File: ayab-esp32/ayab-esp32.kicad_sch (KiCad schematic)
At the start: 22 parts, among them U101 SN74LVC4245

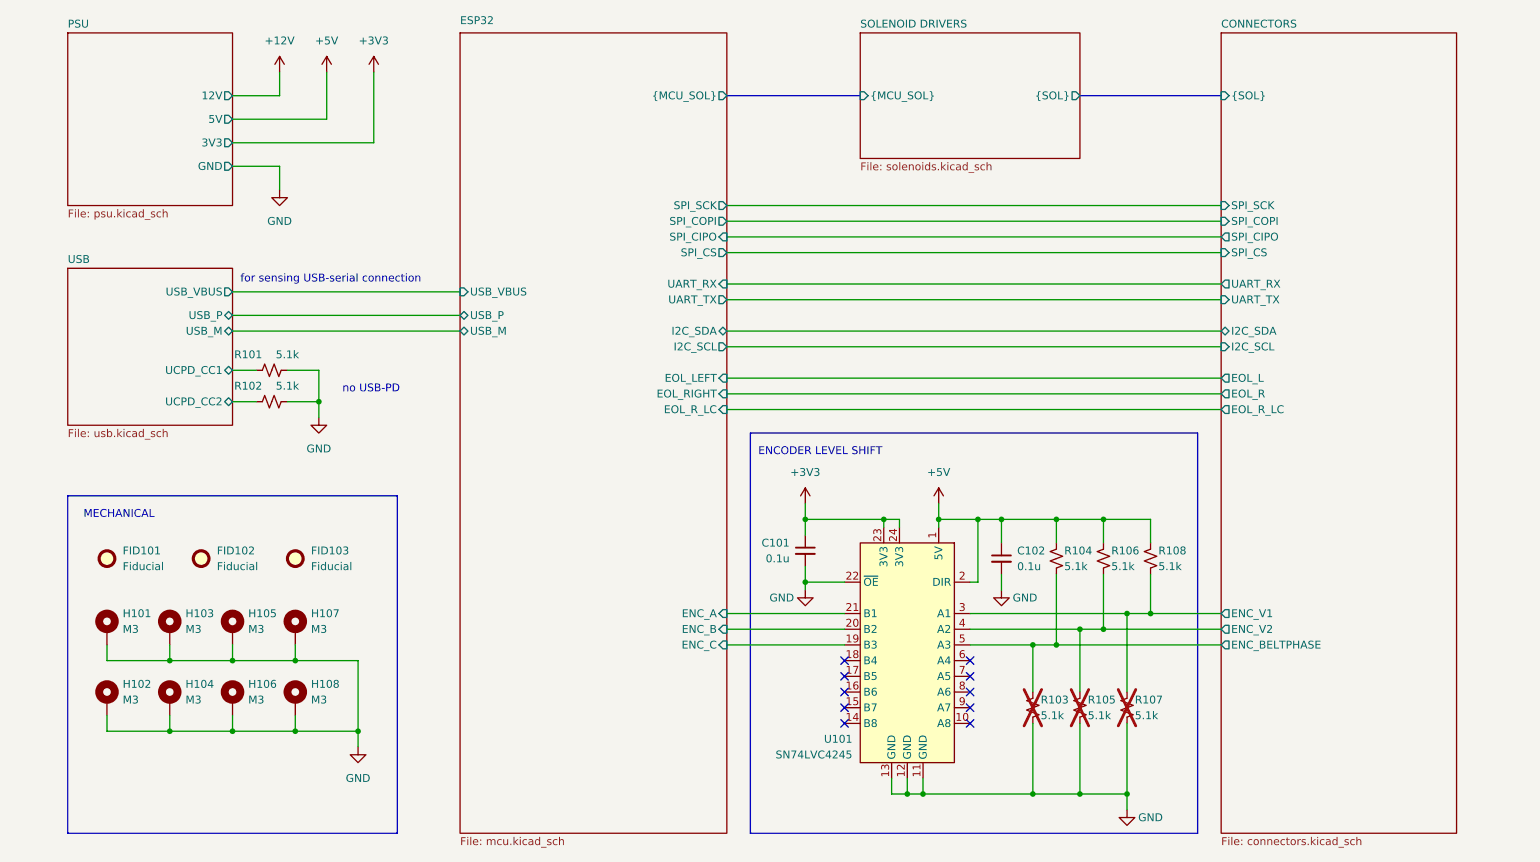
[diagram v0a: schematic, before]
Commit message: fix some comments from jpcornil-git
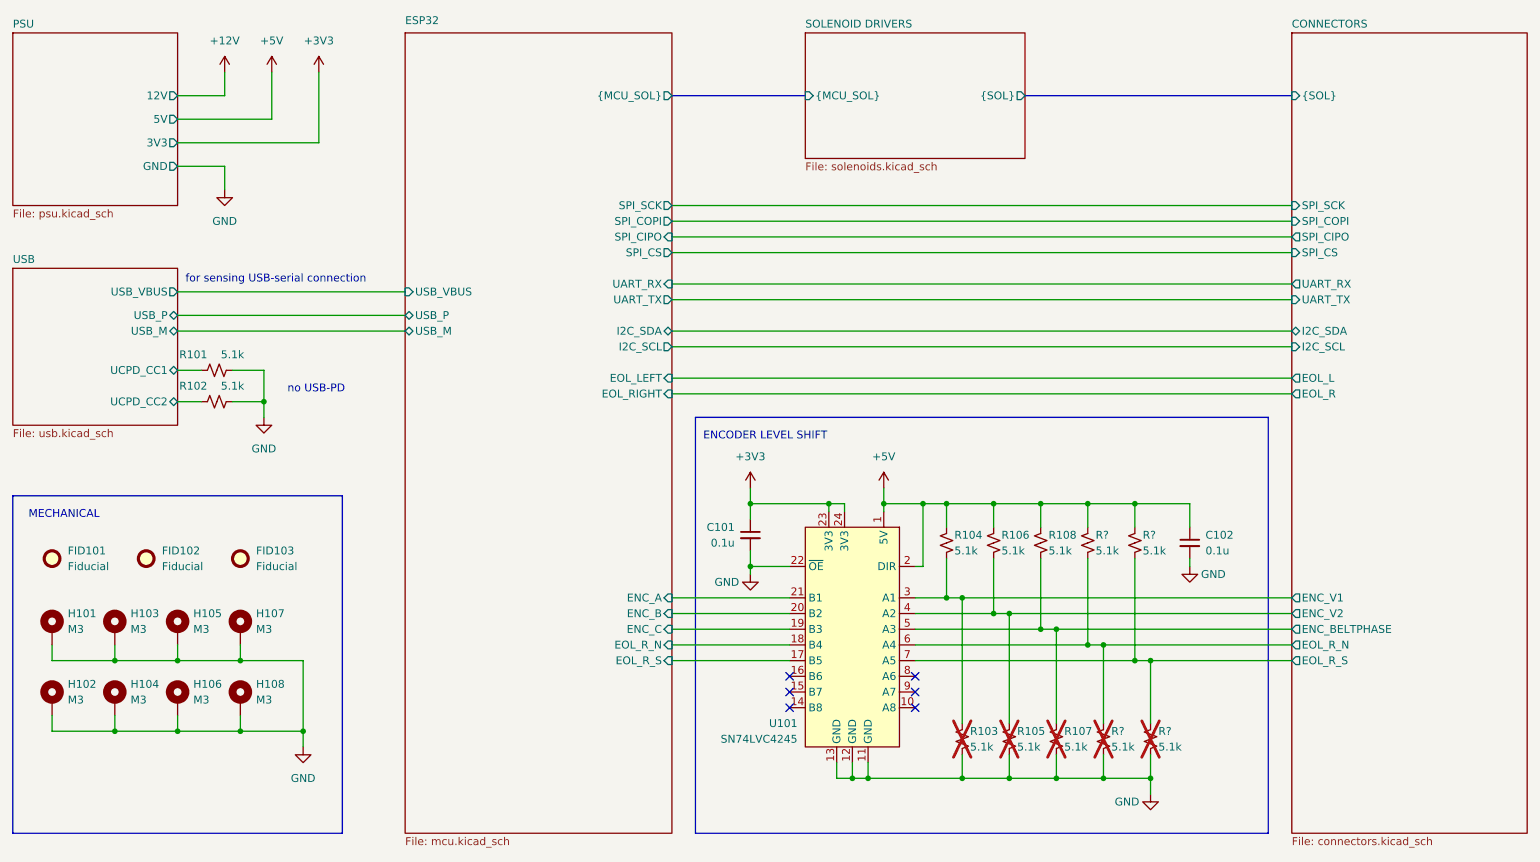
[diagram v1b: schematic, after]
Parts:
- added R? (x4): 5.1k, symbol Device:R_Small_US
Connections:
- net +5V: now also R?.1, R?.1
- net CONNECTORS/ENC_BELTPHASE: now also R107.1, R108.2; no longer R103.1, R104.2
- net CONNECTORS/ENC_V1: now also R103.1, R104.2; no longer R107.1, R108.2
- net GND: now also R?.2, R?.2
- net ESP32/EOL_R_S: now reaches U101.17 (B5)
- net ESP32/EOL_R_N: now reaches U101.18 (B4)
- net CONNECTORS/EOL_R_N: now reaches U101.6 (A4)
- net CONNECTORS/EOL_R_N: now also R?.1, R?.2
- net CONNECTORS/EOL_R_S: now reaches U101.7 (A5)
- net CONNECTORS/EOL_R_S: now also R?.1, R?.2
- no-connect marks 10 -> 6
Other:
- sheet CONNECTORS ports: added EOL_R_N, EOL_R_S; removed EOL_R_LC
- sheet ESP32 ports: added EOL_R_N, EOL_R_S; removed EOL_R_LC
- moved on the sheet: C101, C102, FID101, FID102, FID103, H101, H102, H103, H104, H105, H106, H107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
